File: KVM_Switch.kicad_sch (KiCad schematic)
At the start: 9 parts, among them J1 HDMI_A, J2 HDMI_A, J3 USB_C_Receptacle_USB2.0_16P, J4 USB_C_Receptacle_USB2.0_16P, J5 USB_C_Receptacle_USB2.0_16P, U1 USB2514B_Bi, U2 STM32C011F4Px, U3 TS3USB221AQRSERQ1, U4 HD3SS215RTQR

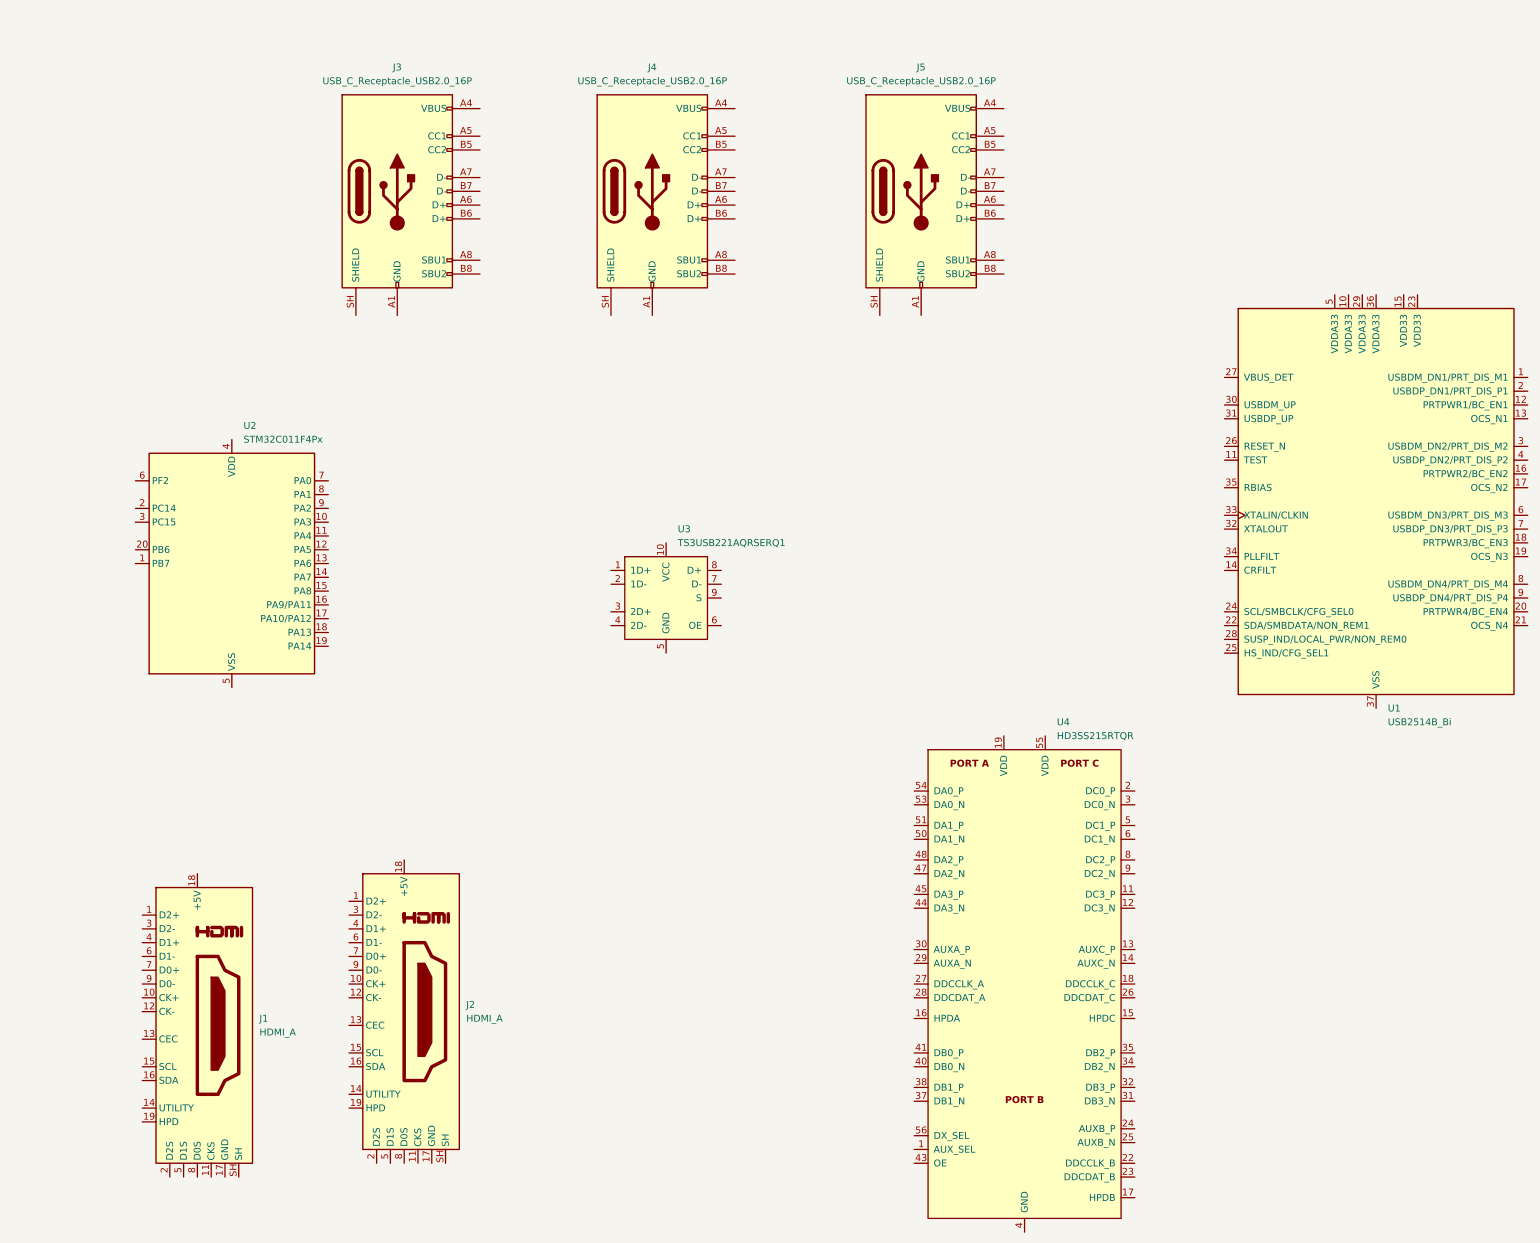
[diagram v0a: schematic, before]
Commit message: Moved stuff armound & added components
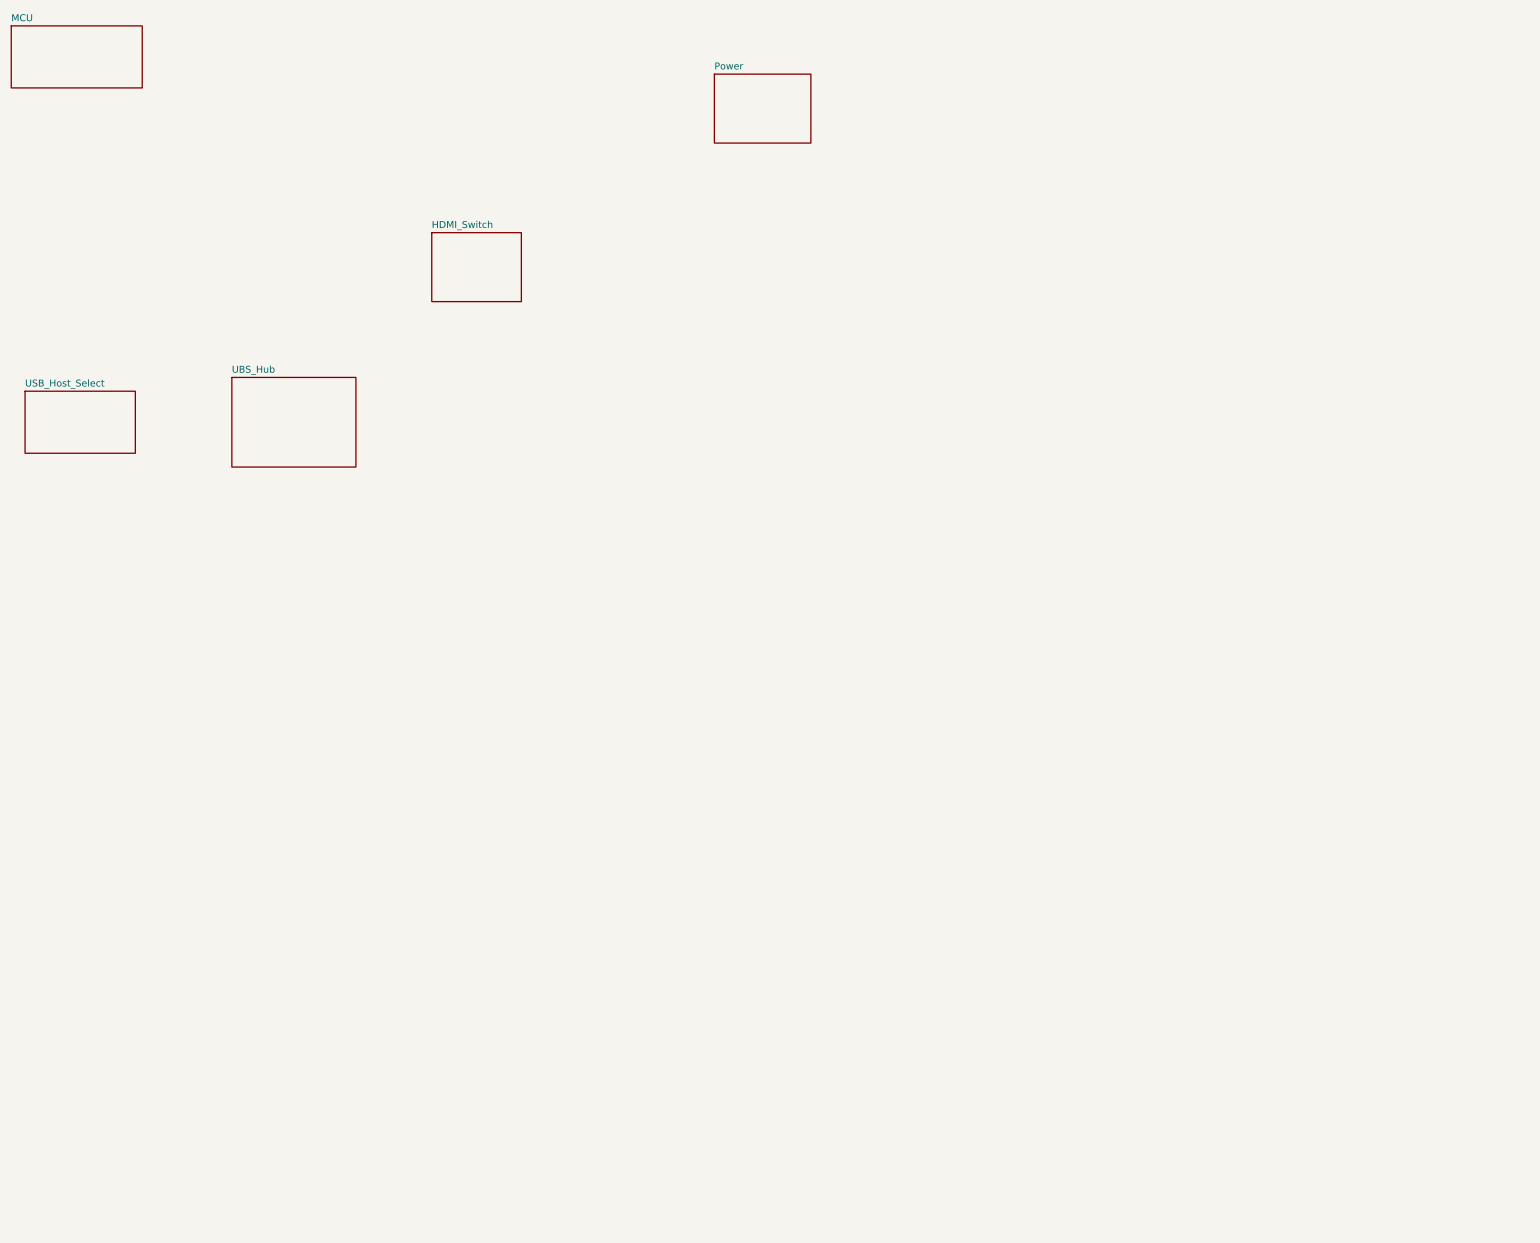
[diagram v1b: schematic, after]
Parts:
- removed J1, J2: HDMI_A, Connector_Video:HDMI_A_Molex_208658-1001_Horizontal, symbol Connector:HDMI_A
- removed J3, J4, J5: USB_C_Receptacle_USB2.0_16P, Connector_USB:USB_C_Receptacle_GCT_USB4105-xx-A_16P_TopMnt_Horizontal, symbol Connector:USB_C_Receptacle_USB2.0_16P
- removed U1: USB2514B_Bi, Package_DFN_QFN:QFN-36-1EP_6x6mm_P0.5mm_EP3.7x3.7mm, symbol Interface_USB:USB2514B_Bi
- removed U2: STM32C011F4Px, Package_SO:TSSOP-20_4.4x6.5mm_P0.65mm, symbol MCU_ST_STM32C0:STM32C011F4Px
- removed U3: TS3USB221AQRSERQ1, TS3USB221AQRSERQ1:TS3USB221AQRSERQ1, symbol TS3USB221AQRSERQ1:TS3USB221AQRSERQ1
- removed U4: HD3SS215RTQR, Package_DFN_QFN:QFN-56-1EP_8x8mm_P0.5mm_EP4.3x4.3mm, symbol HD3SS215RTQR:HD3SS215RTQR
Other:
- added sheet HDMI_Switch (HDMI_Switch.kicad_sch)
- added sheet MCU (MCU.kicad_sch)
- added sheet Power (Power.kicad_sch)
- added sheet UBS_Hub (USB_Hub.kicad_sch)
- added sheet USB_Host_Select (USB_Host_Select.kicad_sch)
